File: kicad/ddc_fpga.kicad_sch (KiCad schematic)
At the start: 36 parts, among them U13 T20Q100F3C3

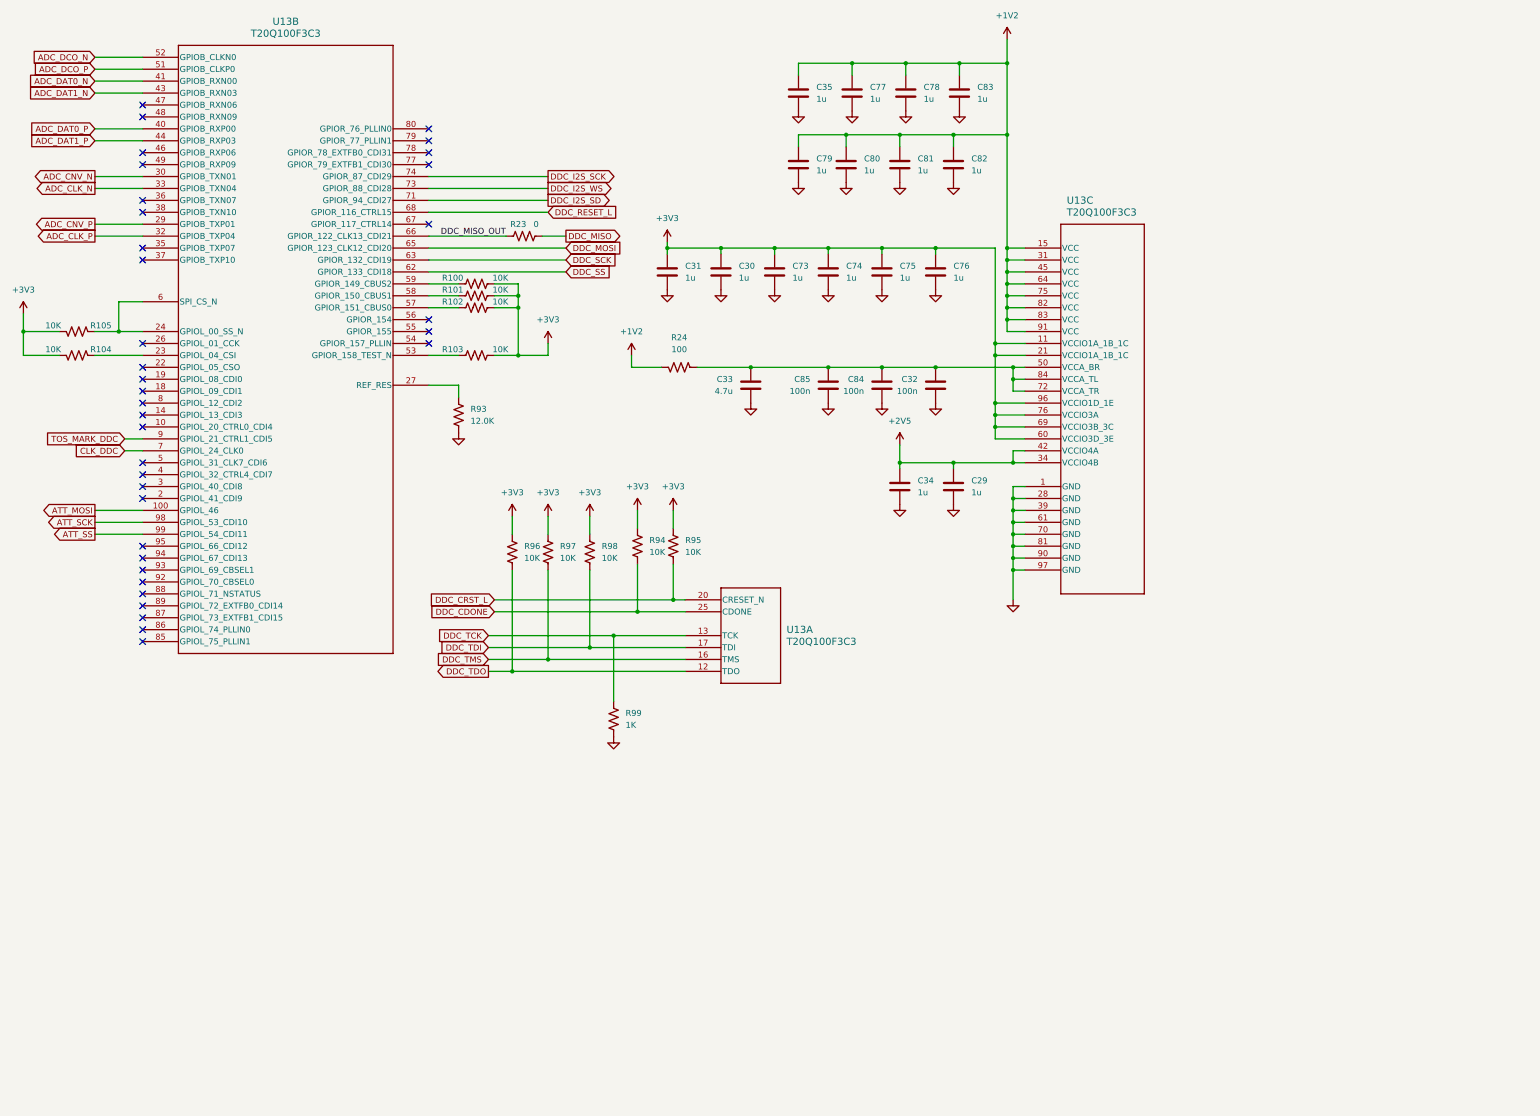
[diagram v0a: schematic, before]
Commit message: add lte radio and various fixes
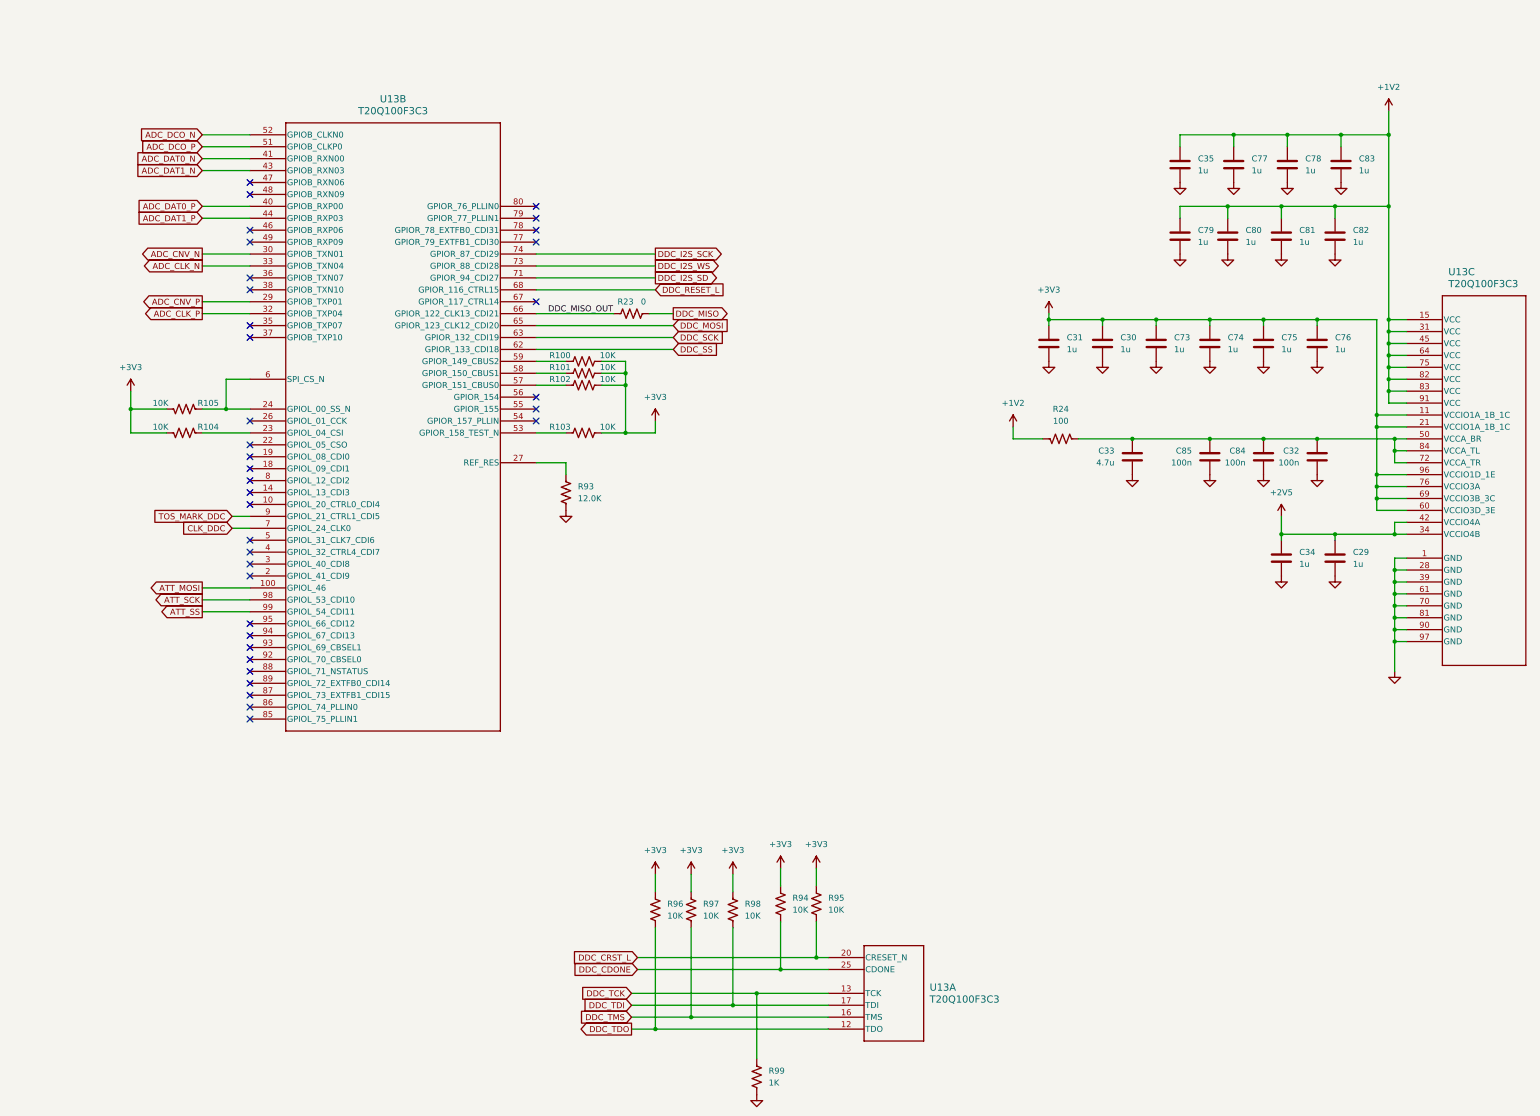
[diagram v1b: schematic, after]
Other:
- moved on the sheet: C29, C30, C31, C32, C33, C34, C35, C73, C74, C75, C76, C77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

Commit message: assign footprints
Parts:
- C29, C30, C31, C32, C33, C34, C35, C73, C74, C75, C76, C77, C78, C79, C80, C81, C82, C83, C84, C85: footprint (none) -> Capacitor_SMD:C_0603_1608Metric_Pad1.08x0.95mm_HandSolder
- R100, R101, R102, R103, R104, R105, R23, R24, R93, R94, R95, R96, R97, R98, R99: footprint (none) -> Resistor_SMD:R_0603_1608Metric_Pad0.98x0.95mm_HandSolder
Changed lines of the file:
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@@
       (effects (font (size 1.27 1.27)) (justify left))
     )
-    (property "Footprint" "" (at 197.866 246.634 90)
+    (property "Footprint" "Resistor_SMD:R_0603_1608Metric_Pad0.98x0.95mm_HandSolder" (at 197.866 246.634 90)
       (effects (font (size 1.27 1.27)) hide)
     )
@@
       (effects (font (size 1.27 1.27)))
     )
-    (property "Footprint" "" (at 160.274 92.964 90)
+    (property "Footprint" "Resistor_SMD:R_0603_1608Metric_Pad0.98x0.95mm_HandSolder" (at 160.274 92.964 90)
       (effects (font (size 1.27 1.27)) hide)
     )
@@
       (effects (font (size 1.27 1.27)))
     )
-    (property "Footprint" "" (at 170.434 82.804 90)
+    (property "Footprint" "Resistor_SMD:R_0603_1608Metric_Pad0.98x0.95mm_HandSolder" (at 170.434 82.804 90)
       (effects (font (size 1.27 1.27)) hide)
     )
@@
       (effects (font (size 1.27 1.27)) (justify left))
     )
-    (property "Footprint" "" (at 309.5752 139.7 0)
+    (property "Footprint" "Capacitor_SMD:C_0603_1608Metric_Pad1.08x0.95mm_HandSolder" (at 309.5752 139.7 0)
       (effects (font (size 1.27 1.27)) hide)
     )
@@
       (effects (font (size 1.27 1.27)))
     )
-    (property "Footprint" "" (at 74.676 103.124 90)
+    (property "Footprint" "Resistor_SMD:R_0603_1608Metric_Pad0.98x0.95mm_HandSolder" (at 74.676 103.124 90)
       (effects (font (size 1.27 1.27)) hide)
     )
@@
       (effects (font (size 1.27 1.27)) (justify left))
     )
-    (property "Footprint" "" (at 210.566 209.804 90)
+    (property "Footprint" "Resistor_SMD:R_0603_1608Metric_Pad0.98x0.95mm_HandSolder" (at 210.566 209.804 90)
       (effects (font (size 1.27 1.27)) hide)
     )
@@
       (effects (font (size 1.27 1.27)) (justify left))
     )
-    (property "Footprint" "" (at 294.3352 93.98 0)
+    (property "Footprint" "Capacitor_SMD:C_0603_1608Metric_Pad1.08x0.95mm_HandSolder" (at 294.3352 93.98 0)
       (effects (font (size 1.27 1.27)) hide)
     )
@@
       (effects (font (size 1.27 1.27)))
     )
-    (property "Footprint" "" (at 160.274 98.044 90)
+    (property "Footprint" "Resistor_SMD:R_0603_1608Metric_Pad0.98x0.95mm_HandSolder" (at 160.274 98.044 90)
       (effects (font (size 1.27 1.27)) hide)
     )
@@
       (effects (font (size 1.27 1.27)) (justify left))
     )
-    (property "Footprint" "" (at 305.7652 93.98 0)
+    (property "Footprint" "Capacitor_SMD:C_0603_1608Metric_Pad1.08x0.95mm_HandSolder" (at 305.7652 93.98 0)
       (effects (font (size 1.27 1.27)) hide)
     )
@@
       (effects (font (size 1.27 1.27)) (justify left))
     )
-    (property "Footprint" "" (at 292.4048 118.11 0)
+    (property "Footprint" "Capacitor_SMD:C_0603_1608Metric_Pad1.08x0.95mm_HandSolder" (at 292.4048 118.11 0)
       (effects (font (size 1.27 1.27)) hide)
     )
@@
       (effects (font (size 1.27 1.27)) (justify left))
     )
-    (property "Footprint" "" (at 309.5752 71.12 0)
+    (property "Footprint" "Capacitor_SMD:C_0603_1608Metric_Pad1.08x0.95mm_HandSolder" (at 309.5752 71.12 0)
       (effects (font (size 1.27 1.27)) hide)
     )
@@
       (effects (font (size 1.27 1.27)) (justify left))
     )
-    (property "Footprint" "" (at 282.9052 93.98 0)
+    (property "Footprint" "Capacitor_SMD:C_0603_1608Metric_Pad1.08x0.95mm_HandSolder" (at 282.9052 93.98 0)
       (effects (font (size 1.27 1.27)) hide)
     )
@@
       (effects (font (size 1.27 1.27)))
     )
-    (property "Footprint" "" (at 160.274 108.204 90)
+    (property "Footprint" "Resistor_SMD:R_0603_1608Metric_Pad0.98x0.95mm_HandSolder" (at 160.274 108.204 90)
       (effects (font (size 1.27 1.27)) hide)
     )
@@
       (effects (font (size 1.27 1.27)) (justify left))
     )
-    (property "Footprint" "" (at 271.4752 93.98 0)
+    (property "Footprint" "Capacitor_SMD:C_0603_1608Metric_Pad1.08x0.95mm_HandSolder" (at 271.4752 93.98 0)
       (effects (font (size 1.27 1.27)) hide)
     )
@@
       (effects (font (size 1.27 1.27)) (justify left))
     )
-    (property "Footprint" "" (at 321.0052 139.7 0)
+    (property "Footprint" "Capacitor_SMD:C_0603_1608Metric_Pad1.08x0.95mm_HandSolder" (at 321.0052 139.7 0)
       (effects (font (size 1.27 1.27)) hide)
     )
@@
       (effects (font (size 1.27 1.27)) (justify left))
     )
-    (property "Footprint" "" (at 321.0052 71.12 0)
+    (property "Footprint" "Capacitor_SMD:C_0603_1608Metric_Pad1.08x0.95mm_HandSolder" (at 321.0052 71.12 0)
       (effects (font (size 1.27 1.27)) hide)
     )
@@
       (effects (font (size 1.27 1.27)) (justify left))
     )
-    (property "Footprint" "" (at 183.896 211.074 90)
+    (property "Footprint" "Resistor_SMD:R_0603_1608Metric_Pad0.98x0.95mm_HandSolder" (at 183.896 211.074 90)
       (effects (font (size 1.27 1.27)) hide)
     )
@@
       (effects (font (size 1.27 1.27)) (justify left))
     )
-    (property "Footprint" "" (at 317.1952 93.98 0)
+    (property "Footprint" "Capacitor_SMD:C_0603_1608Metric_Pad1.08x0.95mm_HandSolder" (at 317.1952 93.98 0)
       (effects (font (size 1.27 1.27)) hide)
     )
@@
       (effects (font (size 1.27 1.27)))
     )
-    (property "Footprint" "" (at 261.366 109.474 90)
+    (property "Footprint" "Resistor_SMD:R_0603_1608Metric_Pad0.98x0.95mm_HandSolder" (at 261.366 109.474 90)
       (effects (font (size 1.27 1.27)) hide)
     )
@@
       (effects (font (size 1.27 1.27)) (justify left))
     )
-    (property "Footprint" "" (at 157.226 122.174 90)
+    (property "Footprint" "Resistor_SMD:R_0603_1608Metric_Pad0.98x0.95mm_HandSolder" (at 157.226 122.174 90)
       (effects (font (size 1.27 1.27)) hide)
     )
@@
       (effects (font (size 1.27 1.27)) (justify left))
     )
-    (property "Footprint" "" (at 322.2752 55.88 0)
+    (property "Footprint" "Capacitor_SMD:C_0603_1608Metric_Pad1.08x0.95mm_HandSolder" (at 322.2752 55.88 0)
       (effects (font (size 1.27 1.27)) hide)
     )
@@
       (effects (font (size 1.27 1.27)) (justify left))
     )
-    (property "Footprint" "" (at 202.946 209.804 90)
+    (property "Footprint" "Resistor_SMD:R_0603_1608Metric_Pad0.98x0.95mm_HandSolder" (at 202.946 209.804 90)
       (effects (font (size 1.27 1.27)) hide)
     )
@@
       (effects (font (size 1.27 1.27)) (justify left))
     )
-    (property "Footprint" "" (at 176.276 211.074 90)
+    (property "Footprint" "Resistor_SMD:R_0603_1608Metric_Pad0.98x0.95mm_HandSolder" (at 176.276 211.074 90)
       (effects (font (size 1.27 1.27)) hide)
     )
@@
       (effects (font (size 1.27 1.27)) (justify left))
     )
-    (property "Footprint" "" (at 298.1452 71.12 0)
+    (property "Footprint" "Capacitor_SMD:C_0603_1608Metric_Pad1.08x0.95mm_HandSolder" (at 298.1452 71.12 0)
       (effects (font (size 1.27 1.27)) hide)
     )
@@
       (effects (font (size 1.27 1.27)) (justify left))
     )
-    (property "Footprint" "" (at 299.4152 55.88 0)
+    (property "Footprint" "Capacitor_SMD:C_0603_1608Metric_Pad1.08x0.95mm_HandSolder" (at 299.4152 55.88 0)
       (effects (font (size 1.27 1.27)) hide)
     )
@@
       (effects (font (size 1.27 1.27)) (justify left))
     )
-    (property "Footprint" "" (at 310.8452 55.88 0)
+    (property "Footprint" "Capacitor_SMD:C_0603_1608Metric_Pad1.08x0.95mm_HandSolder" (at 310.8452 55.88 0)
       (effects (font (size 1.27 1.27)) hide)
     )
@@
       (effects (font (size 1.27 1.27)))
     )
-    (property "Footprint" "" (at 74.676 108.204 90)
+    (property "Footprint" "Resistor_SMD:R_0603_1608Metric_Pad0.98x0.95mm_HandSolder" (at 74.676 108.204 90)
       (effects (font (size 1.27 1.27)) hide)
     )
@@
       (effects (font (size 1.27 1.27)) (justify left))
     )
-    (property "Footprint" "" (at 287.9852 71.12 0)
+    (property "Footprint" "Capacitor_SMD:C_0603_1608Metric_Pad1.08x0.95mm_HandSolder" (at 287.9852 71.12 0)
       (effects (font (size 1.27 1.27)) hide)
     )
@@
       (effects (font (size 1.27 1.27)))
     )
-    (property "Footprint" "" (at 160.274 95.504 90)
+    (property "Footprint" "Resistor_SMD:R_0603_1608Metric_Pad0.98x0.95mm_HandSolder" (at 160.274 95.504 90)
       (effects (font (size 1.27 1.27)) hide)
     )
@@
       (effects (font (size 1.27 1.27)) (justify left))
     )
-    (property "Footprint" "" (at 260.0452 93.98 0)
+    (property "Footprint" "Capacitor_SMD:C_0603_1608Metric_Pad1.08x0.95mm_HandSolder" (at 260.0452 93.98 0)
       (effects (font (size 1.27 1.27)) hide)
     )
@@
       (effects (font (size 1.27 1.27)) (justify left))
     )
-    (property "Footprint" "" (at 303.8348 118.11 0)
+    (property "Footprint" "Capacitor_SMD:C_0603_1608Metric_Pad1.08x0.95mm_HandSolder" (at 303.8348 118.11 0)
       (effects (font (size 1.27 1.27)) hide)
     )
@@
       (effects (font (size 1.27 1.27)) (justify left))
     )
-    (property "Footprint" "" (at 287.9852 55.88 0)
+    (property "Footprint" "Capacitor_SMD:C_0603_1608Metric_Pad1.08x0.95mm_HandSolder" (at 287.9852 55.88 0)
       (effects (font (size 1.27 1.27)) hide)
     )
@@
       (effects (font (size 1.27 1.27)) (justify left))
     )
-    (property "Footprint" "" (at 275.8948 118.11 0)
+    (property "Footprint" "Capacitor_SMD:C_0603_1608Metric_Pad1.08x0.95mm_HandSolder" (at 275.8948 118.11 0)
       (effects (font (size 1.27 1.27)) hide)
     )
@@
       (effects (font (size 1.27 1.27)) (justify left))
     )
-    (property "Footprint" "" (at 315.2648 118.11 0)
+    (property "Footprint" "Capacitor_SMD:C_0603_1608Metric_Pad1.08x0.95mm_HandSolder" (at 315.2648 118.11 0)
       (effects (font (size 1.27 1.27)) hide)
     )
@@
       (effects (font (size 1.27 1.27)) (justify left))
     )
-    (property "Footprint" "" (at 192.786 211.074 90)
-      (effects (font (size 1.27 1.27)) hide)
-    )
+    (property "Footprint" "Resistor_SMD:R_0603_1608Metric_Pad0.98x0.95mm_HandSolder" (at 192.786 211.074 90)
+      (effects (font (size 1.27 1.27)) hide)
+    )
